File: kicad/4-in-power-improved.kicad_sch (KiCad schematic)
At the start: 47 parts, among them J1 USB_C_Receptacle_USB2.0_16P, J2 Bus_PCI_Express_x1, U1 XC6206P332MR, U17 2P SMD 2.54P Jumper, U2 2P SMD 2.54P Jumper, U3 W25Q128JVP, U4 2P SMD 2.54P Jumper, U5 MCP25625T-E/ML, U6 RP2040, X1 ABM8-272-T3, Y1 X322516MLB4SI

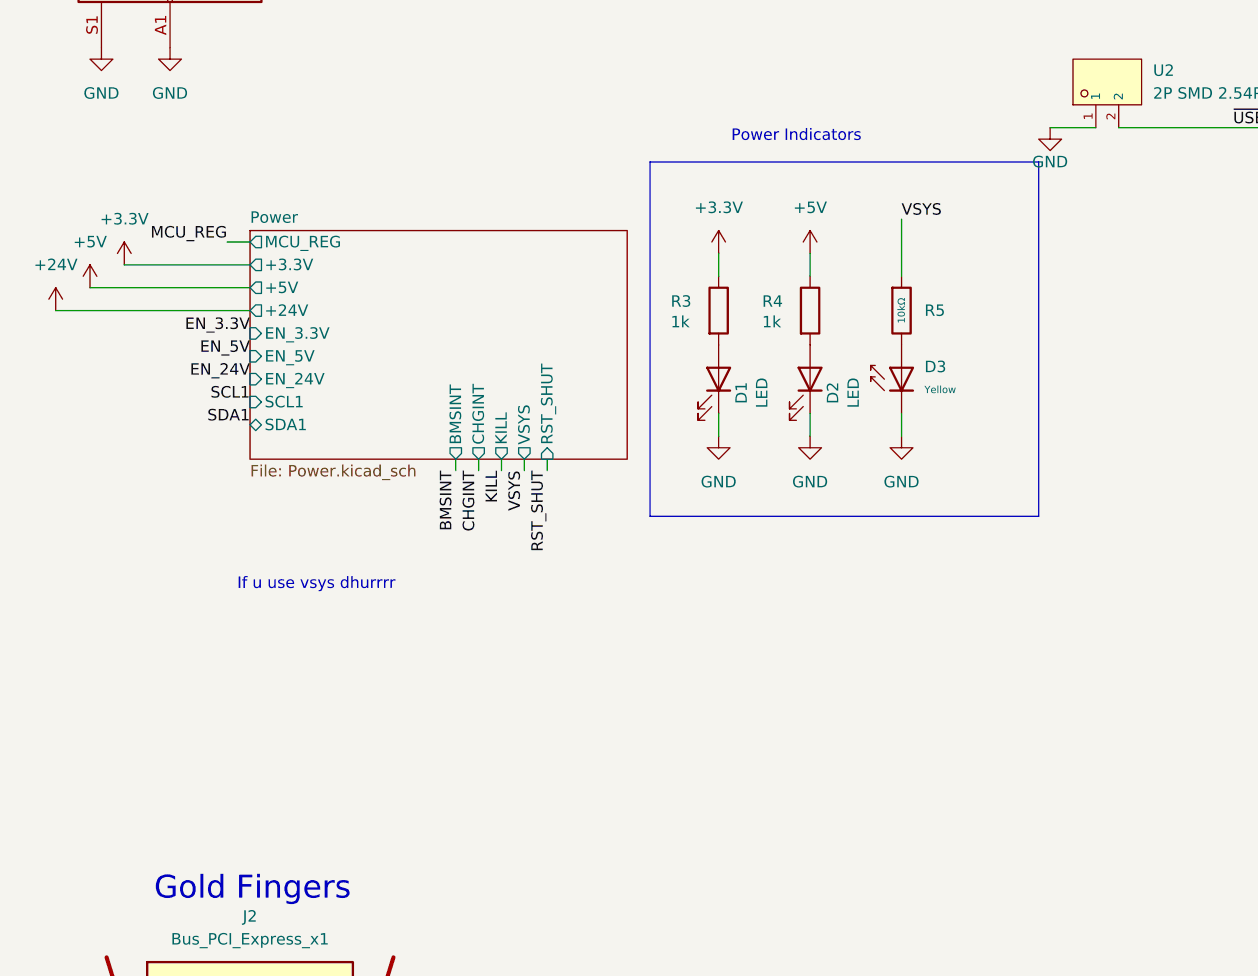
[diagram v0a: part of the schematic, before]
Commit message: Silk screen UI changes
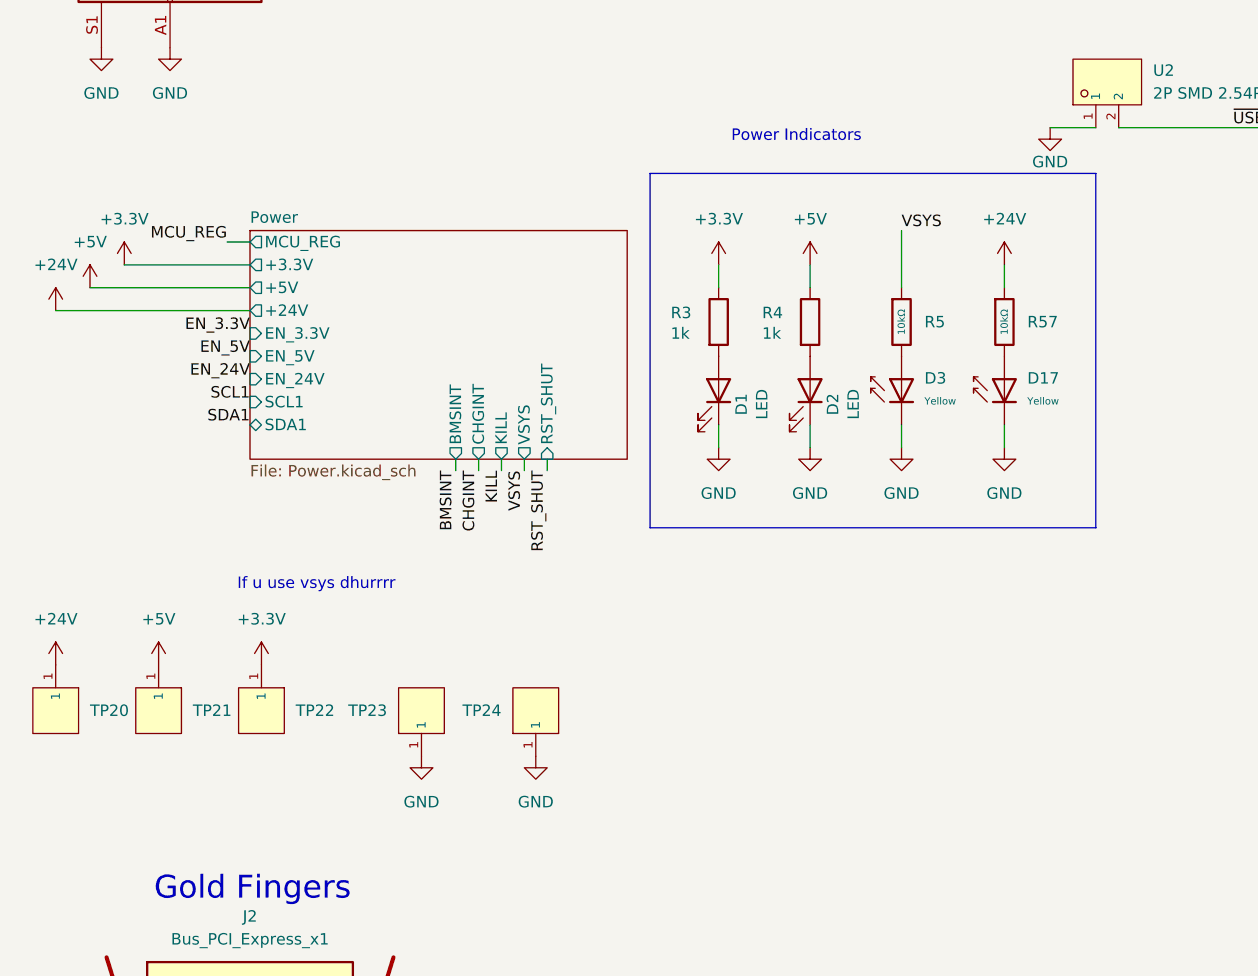
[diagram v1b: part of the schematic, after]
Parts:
- added D17: Yellow, PCM_JLCPCB:D_0603, symbol PCM_JLCPCB-Diodes:LED,0603,Yellow
- added R57: 10kΩ, PCM_JLCPCB:R_0402, symbol 4in-power:0402,10kΩ
- added TP20, TP21, TP22, TP23, TP24: RH-5015, 4in-power:SMD_RH-5015, symbol 4in-power:RH-5015
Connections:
- net +24V: now also R57.1, TP20.1
- net +3.3V: now also TP22.1
- net +5V: now also TP21.1
- net GND: now also D17.1, TP23.1, TP24.1
- new net: D17.2, R57.2
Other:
- moved on the sheet: D1, D2, D3, R3, R4, R5
